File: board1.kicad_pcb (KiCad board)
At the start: 2 copper layers, 101.2 x 101.2 mm, 24 parts, among them J6 XT30 Male Connector, U1 BNO085, U2 Teensy_4.0, U3 Raspberry_PI_Zero_W, U4 D24V50F5

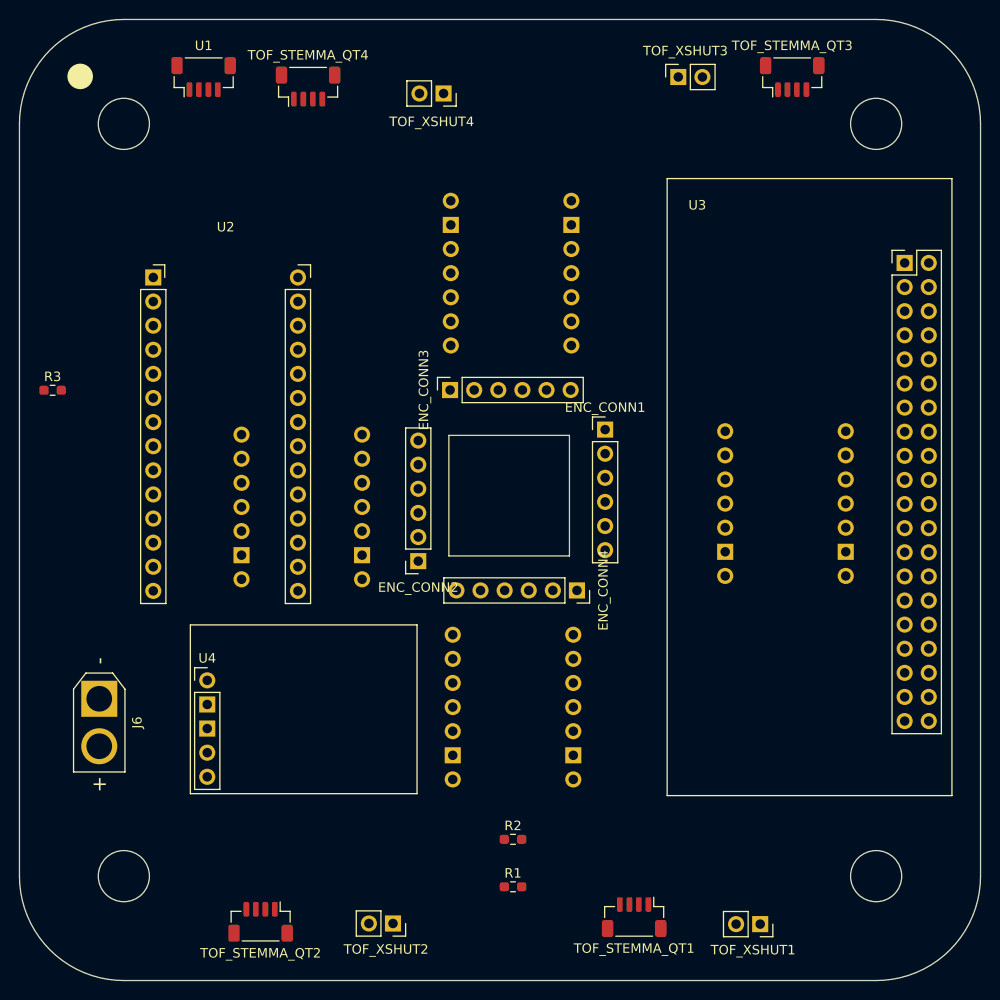
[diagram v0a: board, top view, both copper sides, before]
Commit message: preliminary routing of traces
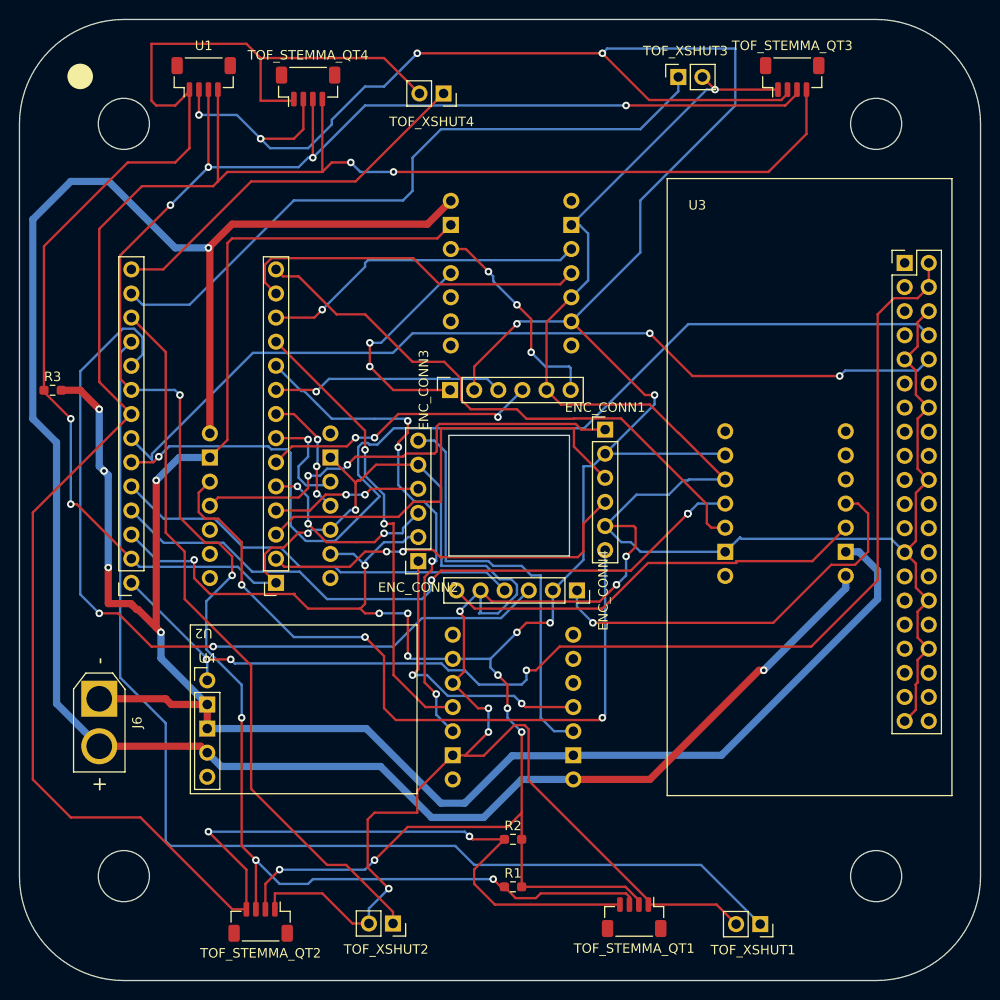
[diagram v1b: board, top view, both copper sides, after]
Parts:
- moved U2 43.7 mm to (119.0, 123.0), turned to 180 degrees
- moved MC1 27.3 mm to (126.0, 95.7), turned to 180 degrees
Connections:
- U2 pad 4: unconnected-(U2-Pad4) -> GNDREF
- U3 pad 14: unconnected-(U3-Pad14) -> GNDREF
- U3 pad 20: unconnected-(U3-Pad20) -> GNDREF
- U3 pad 25: unconnected-(U3-Pad25) -> GNDREF
- U3 pad 30: unconnected-(U3-Pad30) -> GNDREF
- U3 pad 34: unconnected-(U3-Pad34) -> GNDREF
- U3 pad 39: unconnected-(U3-Pad39) -> GNDREF
- U3 pad 4: unconnected-(U3-Pad4) -> /5V
- U3 pad 9: unconnected-(U3-Pad9) -> GNDREF
- U4 pad 3: unconnected-(U4-Pad3) -> /BATTERY_GROUND
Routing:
- net GNDREF: track 0.00 -> 488.3 mm, vias 0 -> 11
- net /3V3_Teensy: track 0.00 -> 342.8 mm, vias 0 -> 18
- net /SCL_LINE: track 0.00 -> 257.0 mm, vias 0 -> 4
- net /12V: track 0.00 -> 221.6 mm, vias 0 -> 2
- net /BATTERY_GROUND: track 0.00 -> 216.9 mm, vias 0 -> 5
- net /SDA_LINE: track 0.00 -> 216.5 mm, vias 0 -> 9
- net /5V: track 0.00 -> 127.9 mm, vias 0 -> 3
- net /TOF_1_XSHUT: track 0.00 -> 121.3 mm
- net /UART TXD (R PI): track 0.00 -> 109.7 mm, vias 0 -> 1
- net /UART RXD (R PI): track 0.00 -> 93.4 mm, vias 0 -> 2
- net /ENC_4_PINB: track 0.00 -> 87.8 mm, vias 0 -> 2
- net /MOTOR_1_PIN1: track 0.00 -> 79.0 mm, vias 0 -> 3
- net /TOF_2_XSHUT: track 0.00 -> 76.4 mm
- net /MC4_PWM2: track 0.00 -> 71.2 mm, vias 0 -> 3
- net /TOF_3_XSHUT: track 0.00 -> 71.0 mm
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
